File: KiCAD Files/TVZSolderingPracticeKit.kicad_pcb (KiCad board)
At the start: 2 copper layers, 100 x 100 mm, 50 parts, among them J1 Barrel Jack, J2 Conn_01x05_Pin, J3 Conn_01x05_Socket, J4 Conn_01x03_Pin, J5 Conn_01x03_Pin, SW1 SW_Push, SW10 POWER, SW11 C/D, SW2 SW_Push, SW3 SW_Push, SW4 SW_Push, SW5 SW_Push, SW6 SW_Push, SW7 SW_Push, SW8 SW_Push, U1 NE555P

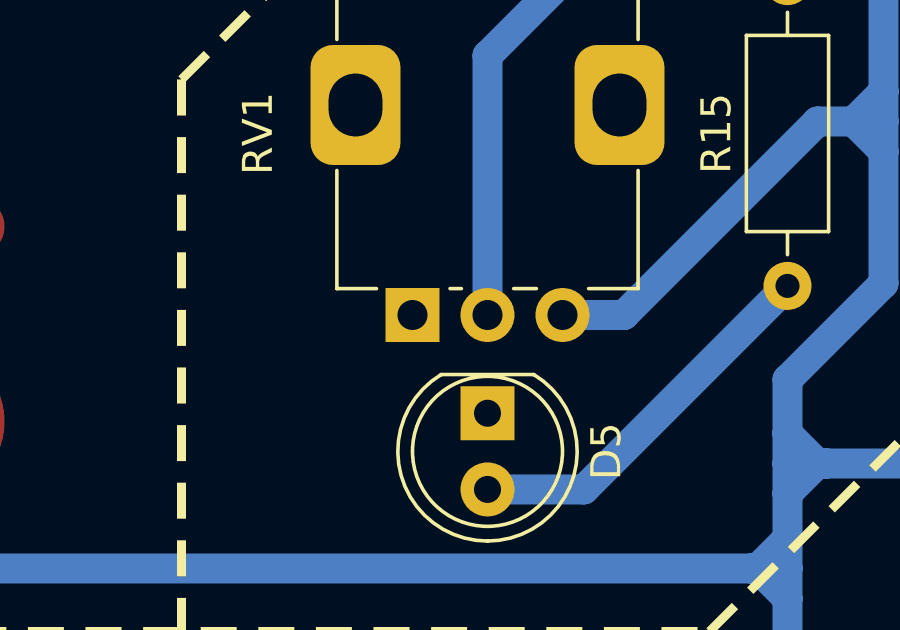
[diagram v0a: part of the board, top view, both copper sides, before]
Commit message: update
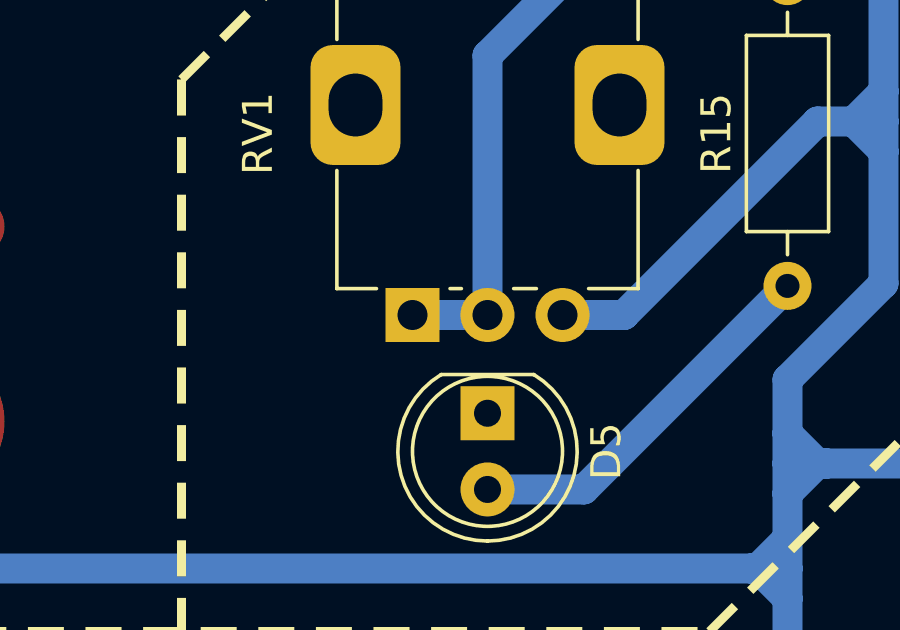
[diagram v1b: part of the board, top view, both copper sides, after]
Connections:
- RV1 pad 1: unconnected-(RV1-Pad1) -> Net-(R15-Pad2)
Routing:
- net Net-(R15-Pad2): track 19.7 -> 22.2 mm
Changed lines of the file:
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@@
 	(net 67 "unconnected-(TP1-Pad1)")
 	(net 68 "unconnected-(TP2-Pad1)")
-	(net 69 "unconnected-(RV1-Pad1)")
-	(net 70 "Net-(D5-A)")
-	(net 71 "Net-(R15-Pad2)")
+	(net 69 "Net-(D5-A)")
+	(net 70 "Net-(R15-Pad2)")
 	(footprint "Resistor_THT:R_Axial_DIN0207_L6.3mm_D2.5mm_P2.54mm_Vertical"
 		(layer "F.Cu")
@@
 		(tags "Through hole pin header THT 1x03 2.54mm single row")
 		(property "Reference" "J5"
-			(at 0 -2.38 180)
+			(at 0 -2.38 0)
 			(layer "F.SilkS")
 			(effects
@@
 			)
 		)
+		(property "TME Part Number" "ZL201-03G"
+			(at 0 0 270)
+			(unlocked yes)
+			(layer "F.Fab")
+			(hide yes)
+			(effects
+				(font
+					(size 1 1)
+					(thickness 0.15)
+				)
+			)
+		)
 		(property ki_fp_filters "Connector*:*_1x??_*")
 		(sheetname "/")
@@
 		)
 		(embedded_fonts no)
-		(model "${KICAD9_3DMODEL_DIR}/Connector_PinHeader_2.54mm.3dshapes/PinHeader_1x03_P2.54mm_Vertical.wrl"
+		(model "${KIPRJMOD}/Component3DModels/pinheader 1x3 and 1 jumper pullback black.step"
 			(offset
-				(xyz 0 0 0)
+				(xyz -11 17.5 0)
 			)
 			(scale
@@
 			)
 			(rotate
-				(xyz 0 0 0)
+				(xyz -0 -0 90)
 			)
 		)
@@
 			(layers "*.Cu" "*.Mask")
 			(remove_unused_layers no)
-			(net 69 "unconnected-(RV1-Pad1)")
+			(net 70 "Net-(R15-Pad2)")
 			(pinfunction "1")
-			(pintype "passive+no_connect")
+			(pintype "passive")
 		)
 		(pad "2" thru_hole circle
@@
 			(layers "*.Cu" "*.Mask")
 			(remove_unused_layers no)
-			(net 71 "Net-(R15-Pad2)")
+			(net 70 "Net-(R15-Pad2)")
 			(pinfunction "2")
 			(pintype "passive")
@@
 		(tags "Through hole pin header THT 1x03 2.54mm single row")
 		(property "Reference" "J4"
-			(at 0 -2.38 180)
+			(at 0 -2.38 0)
 			(layer "F.SilkS")
 			(effects
@@
 			)
 		)
+		(property "TME Part Number" "ZL201-03G"
+			(at 0 0 270)
+			(unlocked yes)
+			(layer "F.Fab")
+			(hide yes)
+			(effects
+				(font
+					(size 1 1)
+					(thickness 0.15)
+				)
+			)
+		)
 		(property ki_fp_filters "Connector*:*_1x??_*")
 		(sheetname "/")
@@
 		)
 		(embedded_fonts no)
-		(model "${KICAD9_3DMODEL_DIR}/Connector_PinHeader_2.54mm.3dshapes/PinHeader_1x03_P2.54mm_Vertical.wrl"
+		(model "${KIPRJMOD}/Component3DModels/pinheader 1x3 and 1 jumper pullback.stp"
 			(offset
-				(xyz 0 0 0)
+				(xyz -11 17.5 0)
 			)
 			(scale
@@
 			)
 			(rotate
-				(xyz 0 0 0)
+				(xyz -0 -0 90)
 			)
 		)
@@
 		(tags "LED")
 		(property "Reference" "D3"
-			(at 1.27 4.3 180)
+			(at 1.27 4.3 0)
 			(layer "F.SilkS")
 			(effects
@@
 		)
 		(embedded_fonts no)
-		(model "${KICAD9_3DMODEL_DIR}/LED_THT.3dshapes/LED_D5.0mm.wrl"
+		(model "${KIPRJMOD}/Component3DModels/LED_Round_Yellow_D5.0mm.step"
 			(offset
 				(xyz 0 0 0)
@@
 			(layers "*.Cu" "*.Mask")
 			(remove_unused_layers no)
-			(net 70 "Net-(D5-A)")
+			(net 69 "Net-(D5-A)")
 			(pinfunction "A")
 			(pintype "passive")
 		)
 		(embedded_fonts no)
-		(model "${KICAD9_3DMODEL_DIR}/LED_THT.3dshapes/LED_D5.0mm.wrl"
+		(model "${KIPRJMOD}/Component3DModels/LED_Round_Clear_D5.0mm.step"
 			(offset
 				(xyz 0 0 0)
@@
 			)
 		)
+		(property "TME Part Number" "PH1RB-40-UA"
+			(at 0 0 0)
+			(unlocked yes)
+			(layer "F.Fab")
+			(hide yes)
+			(effects
+				(font
+					(size 1 1)
+					(thickness 0.15)
+				)
+			)
+		)
 		(property ki_fp_filters "Connector*:*_1x??_*")
 		(sheetname "/")
@@
 			(layers "*.Cu" "*.Mask")
 			(remove_unused_layers no)
-			(net 70 "Net-(D5-A)")
+			(net 69 "Net-(D5-A)")
 			(pintype "passive")
 		)
@@
 			(layers "*.Cu" "*.Mask")
 			(remove_unused_layers no)
-			(net 71 "Net-(R15-Pad2)")
+			(net 70 "Net-(R15-Pad2)")
 			(pintype "passive")
 		)
@@
 		(tags "LED")
 		(property "Reference" "D4"
-			(at 1.275 4.3 180)
+			(at 1.275 4.3 0)
 			(layer "F.SilkS")
 			(effects
@@
 		)
 		(embedded_fonts no)
-		(model "${KICAD9_3DMODEL_DIR}/LED_THT.3dshapes/LED_D5.0mm.wrl"
+		(model "${KIPRJMOD}/Component3DModels/LED_Round_Green1_D5.0mm.step"
 			(offset
 				(xyz 0 0 0)
@@
 		(sheetname "/")
 		(sheetfile "TVZSolderingPracticeKit.kicad_sch")
-		(attr board_only exclude_from_pos_files)
+		(attr board_only exclude_from_pos_files exclude_from_bom)
 		(fp_text user "${REFERENCE}"
 			(at 0 4 270)
@@
 			)
 		)
+		(property "TME Part Number" "ZL262-5SG"
+			(at 0 0 270)
+			(unlocked yes)
+			(layer "F.Fab")
+			(hide yes)
+			(effects
+				(font
+					(size 1 1)
+					(thickness 0.15)
+				)
+			)
+		)
 		(property ki_fp_filters "Connector*:*_1x??_*")
 		(sheetname "/")
@@
 		(sheetname "/")
 		(sheetfile "TVZSolderingPracticeKit.kicad_sch")
-		(attr board_only exclude_from_pos_files)
+		(attr board_only exclude_from_pos_files exclude_from_bom)
 		(fp_text user "${REFERENCE}"
 			(at 0 4 270)
@@
 		)
 	)
+	(dimension
+		(type orthogonal)
+		(layer "User.1")
+		(pts
+			(xy 50 84.5) (xy 150 84.5)
+		)
+		(height -8.9)
+		(orientation 0)
+		(format
+			(prefix "")
+			(suffix "")
+			(units 3)
+			(units_format 0)
+			(precision 4)
+			(suppress_zeroes yes)
+		)
+		(style
+			(thickness 0.1)
+			(arrow_length 1.27)
+			(text_position_mode 0)
+			(arrow_direction outward)
+			(extension_height 0.58642)
+			(extension_offset 0.5)
+			(keep_text_aligned yes)
+		)
+		(gr_text "100"
+			(at 100 73.2 0)
+			(layer "User.1")
+			(effects
+				(font
+					(size 2 2)
+					(thickness 0.4)
+					(bold yes)
+				)
+			)
+		)
+	)
+	(dimension
+		(type orthogonal)
+		(layer "User.1")
+		(pts
+			(xy 146 80.5) (xy 146 180.5)
+		)
+		(height 10.4)
+		(orientation 1)
+		(format
+			(prefix "")
+			(suffix "")
+			(units 3)
+			(units_format 0)
+			(precision 4)
+			(suppress_zeroes yes)
+		)
+		(style
+			(thickness 0.1)
+			(arrow_length 1.27)
+			(text_position_mode 0)
+			(arrow_direction outward)
+			(extension_height 0.58642)
+			(extension_offset 0.5)
+			(keep_text_aligned yes)
+		)
+		(gr_text "100"
+			(at 154 130.5 90)
+			(layer "User.1")
+			(effects
+				(font
+					(size 2 2)
+					(thickness 0.4)
+					(bold yes)
+				)
+			)
+		)
+	)
 	(segment
 		(start 147.25 167.88)
@@
 		(width 1)
 		(layer "B.Cu")
-		(net 70)
+		(net 69)
 	)
 	(segment
@@
 		(width 1)
 		(layer "B.Cu")
+		(net 69)
+	)
+	(segment
+		(start 91.7 118.05)
+		(end 94.2 118.05)
+		(width 1)
+		(layer "B.Cu")
 		(net 70)
 	)
@@
 		(width 1)
 		(layer "B.Cu")
-		(net 71)
+		(net 70)
 	)
 	(segment
@@
 		(width 1)
 		(layer "B.Cu")
-		(net 71)
+		(net 70)
 	)
 	(segment
@@
 		(width 1)
 		(layer "B.Cu")
-		(net 71)
+		(net 70)
 	)
 	(zone
